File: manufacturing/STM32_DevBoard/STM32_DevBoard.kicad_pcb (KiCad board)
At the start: 4 copper layers, 60 x 50 mm, 99 parts, among them J1 CAN, J10 I2C, J11 PWM0, J12 Conn_01x03_Pin, J3 Conn_01x03_Pin, J5 USB_A, J6 SWD, J8 SPI/UART, J9 SPI_NSS/GPIO, SW1 SW_SPDT, SW2 SW_Omron_B3FS, SW3 EEPROM_WP, U1 MPU-6050, U2 SHTC3, U3 STM32F405RGT6, U4 AT24C256, U5 USBLC6-2, U6 SN65HVD230, U7 USBLC6-2, U8 LMR16006YQ3, Y1 25MHz 12pF

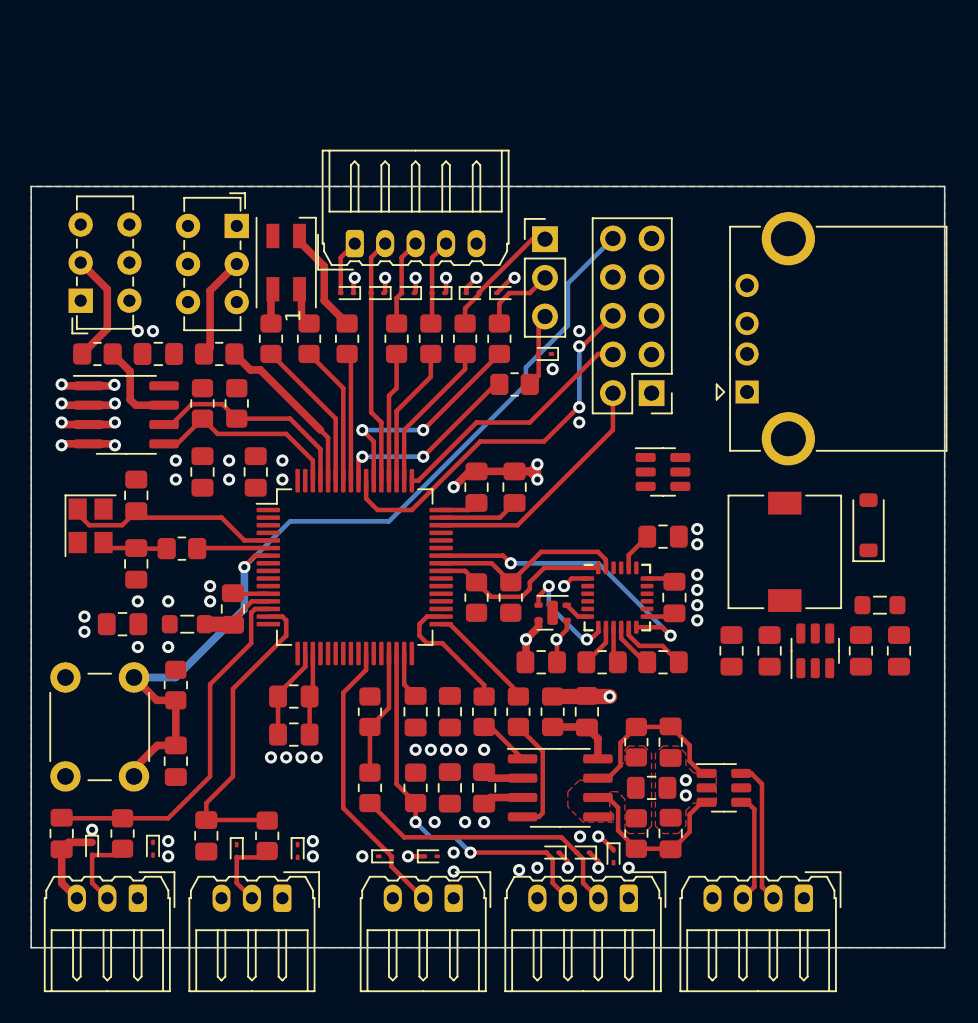
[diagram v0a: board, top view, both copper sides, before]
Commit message: update Board Revision 0
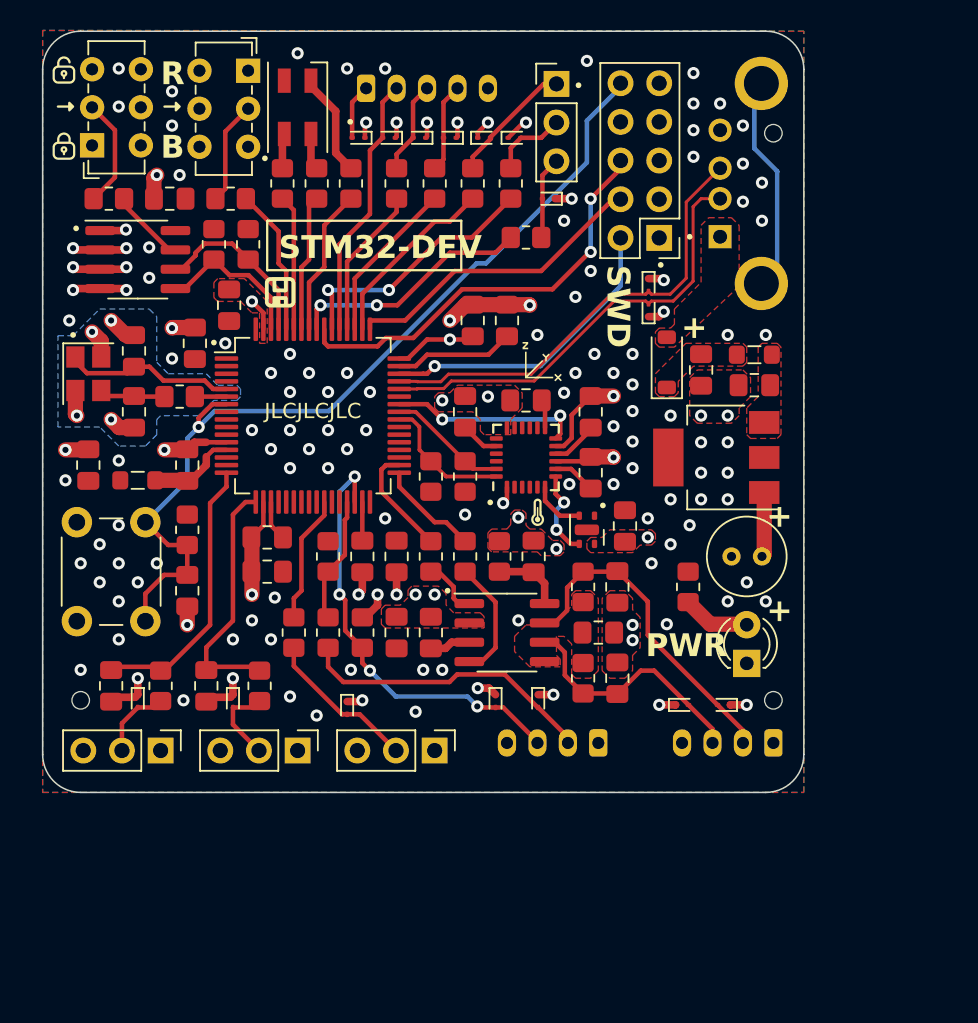
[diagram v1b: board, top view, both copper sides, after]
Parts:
- removed C32: 100n, Capacitor_SMD:C_0805_2012Metric_Pad1.18x1.45mm_HandSolder
- removed C34: 10u, Capacitor_SMD:C_0805_2012Metric_Pad1.18x1.45mm_HandSolder
- removed D14, D16, D19, D23: 3V3, Diode_SMD:D_SOD-923
- removed L1: 3u3, Inductor_SMD:L_7.3x7.3_H4.5
- removed U5, U7: USBLC6-2, Package_TO_SOT_SMD:SOT-23-6
- added C14: 22u, Capacitor_THT:C_Radial_D5.0mm_H7.0mm_P2.00mm, F.Cu at (174.8, 99.3)
- added D15: 3V3, Diode_SMD:D_SOD-923, F.Cu at (171.5, 109.0)
- added D2: GN, LED_THT:LED_D3.0mm, F.Cu at (175.8, 106.3)
- added D20: 3V3, Diode_SMD:D_SOD-923, F.Cu at (174.2, 109.0)
- added D5: 3V3, Diode_SMD:D_SOD-923, F.Cu at (169.3, 81.5)
- added D6: 3V3, Diode_SMD:D_SOD-923, F.Cu at (169.3, 83.1)
- added G***: LOGO, Symbol:Lock_S, F.Cu at (130.9, 72.3)
- added G***: LOGO, Symbol:Temp, F.Cu at (162.0, 96.4)
- added G***: LOGO, Symbol:Gyro_Logo, F.Cu at (162.3, 86.5)
- added G***: LOGO, Symbol:Unlock_S, F.Cu at (130.9, 67.3)
- added G***: LOGO, Symbol:Storage_S, F.Cu at (145.1, 82.0)
- added H4: ~, JLC:JLC_Tooling, F.Cu at (132.0, 108.8)
- added H4: ~, JLC:JLC_Tooling, F.Cu at (177.5, 71.5)
- added H4: ~, JLC:JLC_Tooling, F.Cu at (177.5, 108.8)
- added R11: 1k5, Resistor_SMD:R_0805_2012Metric_Pad1.20x1.40mm_HandSolder, F.Cu at (171.9, 101.3)
- added R17: 10R, Resistor_SMD:R_0805_2012Metric_Pad1.20x1.40mm_HandSolder, F.Cu at (146.0, 104.3)
- C11, C12: value C -> 12p
- FB1, FB2: value xR @ xMHz -> 100R @ 100MHz
- J11: footprint Connector_Molex:Molex_Micro-Latch_53254-0370_1x03_P2.00mm_Horizontal -> Connector_PinHeader_2.54mm:PinHeader_1x03_P2.54mm_Vertical
- J12, J3: value Conn_01x03_Pin -> AGPIO; footprint Connector_Molex:Molex_Micro-Latch_53254-0370_1x03_P2.00mm_Horizontal -> Connector_PinHeader_2.54mm:PinHeader_1x03_P2.54mm_Vertical
- R1: value R -> 0R
- R3: value R -> 10k
- U8: value LMR16006YQ3 -> AMS1117-3.3; footprint Package_TO_SOT_SMD:SOT-23-6 -> Package_TO_SOT_SMD:SOT-223-3_TabPin2
- moved C22 22.6 mm to (172.8, 87.0)
- moved C33 18.8 mm to (176.2, 88.0), turned to 180 degrees
- moved FB2 18.4 mm to (176.2, 86.0), turned to 180 degrees
- moved C15 17.1 mm to (165.5, 89.8), turned to 90 degrees
- moved D24 17.0 mm to (170.5, 86.5)
- moved C20 16.2 mm to (161.2, 89.0), turned to 180 degrees
- moved C16 15.4 mm to (157.2, 89.8), turned to 90 degrees
- moved U8 14.3 mm to (173.8, 92.8), turned to 180 degrees
- moved C19 12.5 mm to (165.5, 93.8), turned to 90 degrees
- moved C13 11.2 mm to (139.0, 101.5)
- moved C3 11.1 mm to (141.8, 82.8)
- moved U1 11.0 mm to (161.2, 92.8), turned to 90 degrees
- moved C9 11.0 mm to (160.0, 83.8)
- moved C2 11.0 mm to (157.8, 83.8)
- moved C6 10.8 mm to (144.2, 100.3)
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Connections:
- C23 pad 1: /Connectors/A_GPIO_1 -> /Connectors/A_GPIO_3
- C25 pad 1: /Connectors/A_GPIO_0 -> /Connectors/A_GPIO_2
- C33 pad 1: /PMU/BUCK_IN -> /PMU/LDO_IN
- D13 pad 2: /Connectors/PWM0 -> Net-(D13-A2)
- FB2 pad 1: /PMU/BUCK_IN -> /PMU/LDO_IN
- J1 pad 2: /Connectors/CAN_CONN+ -> /Connectors/CAN+
- J1 pad 3: /Connectors/CAN_CONN- -> /Connectors/CAN-
- J11 pad 2: /Connectors/PWM0 -> Net-(D13-A2)
- J5 pad 2: /Connectors/USB_CONN- -> /Connectors/USB_D-
- J5 pad 3: /Connectors/USB_CONN+ -> /Connectors/USB_D+
- R10 pad 1: /Connectors/A_GPIO_1 -> /Connectors/A_GPIO_3
- R12 pad 1: /Connectors/A_GPIO_0 -> /Connectors/A_GPIO_2
- U3 pad 14: /Connectors/A_GPIO_0 -> /MCU/A_GPIO_0
- U3 pad 15: /Connectors/A_GPIO_1 -> /MCU/A_GPIO_1
- U3 pad 16: /MCU/A_GPIO_2 -> /Connectors/A_GPIO_2
- U3 pad 17: /MCU/A_GPIO_3 -> /Connectors/A_GPIO_3
- U8 pad 1: /PMU/BUCK_BST -> GND
- U8 pad 2: GND -> +3V3
- U8 pad 3: +3V3 -> /PMU/LDO_IN
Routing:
- net /Connectors/USB_D+: track 0.00 -> 30.0 mm
- net /Connectors/USB_D-: track 0.00 -> 29.3 mm
- net /Connectors/A_GPIO_0: track 24.0 -> 0.00 mm
- net /Connectors/A_GPIO_1: track 20.6 -> 0.00 mm
- net /Connectors/A_GPIO_2: track 0.00 -> 18.4 mm
- net GND: track 69.5 -> 86.5 mm, vias 55 -> 112
- net /Connectors/A_GPIO_3: track 0.00 -> 16.5 mm
- net unconnected-(J5-Shield-Pad5): track 0.00 -> 14.4 mm
- net /Connectors/PWM0: track 18.9 -> 8.40 mm
- net /Connectors/CAN+: track 11.3 -> 21.8 mm
- net Net-(D13-A2): track 0.00 -> 10.2 mm
- net /Connectors/CAN_CONN+: track 9.46 -> 0.00 mm
- net /Connectors/CAN_CONN-: track 7.21 -> 0.00 mm
- net /MCU/IMU_INT: track 19.7 -> 12.7 mm
- net /Connectors/CAN-: track 11.4 -> 16.5 mm
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- added copper zone on F.Cu, net +5V
- added copper zone on F.Cu, net /PMU/LDO_IN
- added copper zone on F.Cu, net /PMU/POST_POL
- added copper zone on B.Cu, net GND
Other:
- board size 60 x 50 mm -> 50 x 50 mm
- board text added: "+"
- board text added: "-"
- board text added: "0"
- board text added: "1"
- board text added: "2"
- board text added: "AIO"
- board text added: "BOOT"
- board text added: "CANH"
- board text added: "CANL"
- board text added: "CS"
- board text added: "JLCJLCJLC"
- board text added: "MISO RX"
- board text added: "MOSI"
- board text added: "PWM"
- board text added: "PWR"
- board text added: "R B"
- board text added: "SCK TX"
- board text added: "SCL"
- board text added: "SDA"
- board text added: "STM32-DEV"
- board text added: "SWD"
- board text added: "WP"
